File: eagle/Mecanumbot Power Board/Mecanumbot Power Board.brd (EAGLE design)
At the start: 100.1 x 74.1 mm, 103 parts, among them J1 AVR_SPI_PRG_6PTH, U1 FT232RL-BASICSSOP, U2 ATMEGA168, X1 USBSMD, Y1 RESONATORSMD

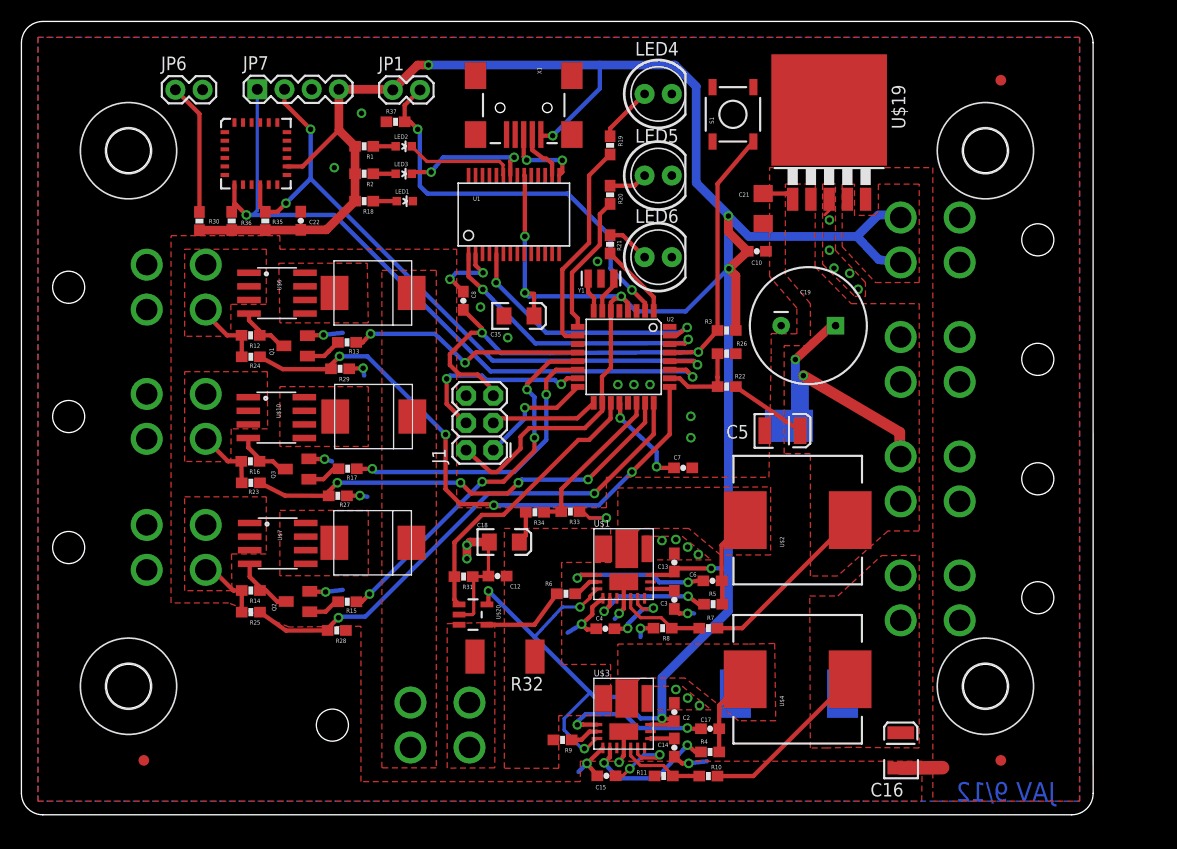
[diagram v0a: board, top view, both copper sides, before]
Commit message: pushing back v2.0 from svn
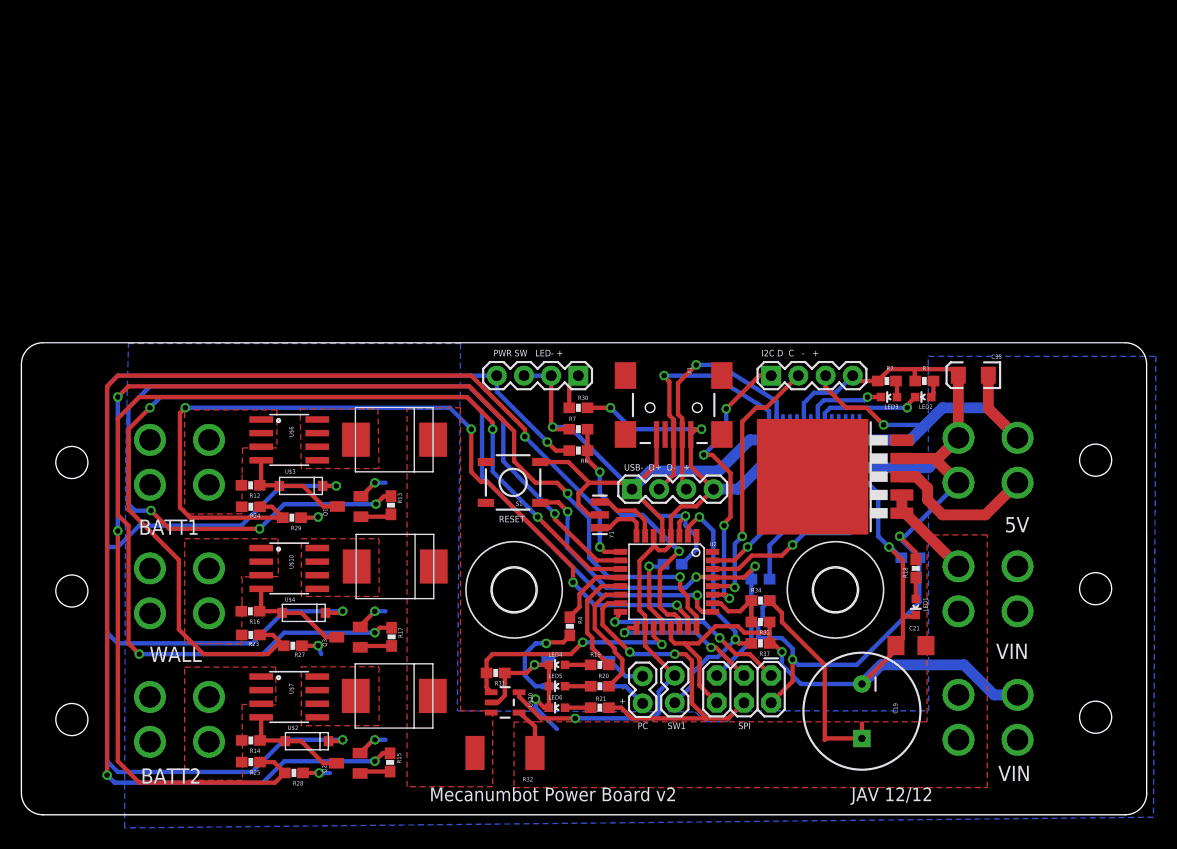
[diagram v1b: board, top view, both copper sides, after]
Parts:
- removed C12, C13, C14, C17, C2, C3, C6: 1uF, SparkFun:0603-CAP
- removed C15, C22, C4: 0.1uF, SparkFun:0603-CAP
- removed C16, C5: 330uF, SparkFun:EIA3528
- removed C18: 68uF, SparkFun:EIA3216
- removed JP4: FIDUCIAL1X2.5, SparkFun:FIDUCIAL-1X2.5
- removed JP6: PWR LED, SparkFun:1X02
- removed R10: 24K, SparkFun:0603-RES
- removed R11, R8: 1K, SparkFun:0603-RES
- removed R22: 10K, SparkFun:0603-RES
- removed R26: 3.3K, SparkFun:0603-RES
- removed R35, R36: 10k, SparkFun:0603-RES
- removed R5: 7.5K, SparkFun:0603-RES
- removed R9: 200K, SparkFun:0603-RES
- removed U$15, U$9: TERMINAL-4MINIFIT-JR, AT-Parts-RJ:MINIFITJR-RGT-4
- removed U$21: SUPERCAPS-LEAD, AT-Parts-RJ:AVX-SUPERCAP-S-LEAD
- removed U$22: HMC6352, SparkFun:LCC24
- removed U$23, U$25: (no value), holes:4,1
- added PC-CTRL: S2, SparkFun:1X02
- JP2: value FIDUCIAL1X2.5 -> USB; device SparkFun:FIDUCIAL-1X2.5 -> SparkFun:1X04
- JP3: value FIDUCIAL1X2.5 -> PWR-CTRL; device SparkFun:FIDUCIAL-1X2.5 -> SparkFun:1X04
- LED3: value Green -> Yellow
- LED4, LED5, LED6: value RED -> Blue; device SparkFun:LED5MM -> SparkFun:LED-0603
- R37: value 10k -> 10K
- R4: value 7.5K -> 330
- R6: value 200K -> 10K
- R7: value 24K -> 3.3K
- U$1: value IR3477 -> CLA230TR-NDSMD; device AT-Parts-RJ:IR3477 -> jav-parts:4-SOP
- U$2, U$4: value 1uH -> BZT52C33-FDICT-ND; device SparkFun:CDRH125 -> jav-parts:SOD-123
- U$3: value IR3477 -> BZT52C33-FDICT-ND; device AT-Parts-RJ:IR3477 -> jav-parts:SOD-123
- moved R18 61.9 mm to (83.5, 23.0), turned to 90 degrees
- moved LED1 60.9 mm to (83.5, 19.4), turned to 180 degrees
- moved JP1 60.7 mm to (61.0, 13.0), turned to 270 degrees
- moved R37 59.4 mm to (69.0, 16.0), turned to 180 degrees
- moved R1 56.7 mm to (84.3, 40.5)
- moved JP7 54.9 mm to (70.0, 41.0)
- moved U$26 54.6 mm to (46.0, 21.0)
- moved LED4 54.1 mm to (50.0, 14.0), turned to 90 degrees
- moved LED2 53.9 mm to (84.2, 39.0), turned to 90 degrees
- moved JP3 53.3 mm to (52.0, 41.0), turned to 180 degrees
- moved R2 52.5 mm to (80.8, 40.5)
- moved JP2 52.1 mm to (57.0, 30.4)
- moved U$2 50.3 mm to (26.6, 6.87), turned to 0 degrees
- moved LED3 49.9 mm to (81.0, 39.0), turned to 90 degrees
- moved LED5 48.6 mm to (50.0, 12.0), turned to 90 degrees
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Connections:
- removed net 12VA: C19.1, C21.1, C5.A, R22.2, R7.2, U$15.3, U$15.4, U$17.3, U$17.4, U$19.1, U$19.2, U$2.2, U$21.PLUS1
- removed net 12VB: C16.A, R10.2, U$16.3, U$16.4, U$4.2
- removed net N$17: R4.1, U$3.2
- removed net N$18: C3.2, U$1.8
- removed net N$19: R6.1, U$1.15
- removed net N$21: R10.1, R11.2, U$3.5
- removed net N$22: C14.2, U$3.8
- removed net N$23: R9.1, U$3.15
- removed net N$24: C15.2, U$3.6
- removed net N$25: C4.2, U$1.6
- removed net N$35: R19.2, U2.10
- removed net N$36: R20.2, U2.9
- removed net N$37: R21.2, U2.1
- removed net N$41: R22.1, R26.2, U2.26
- removed net N$45: JP6.1, R30.2
- removed net POST-DIODE: U$11.P$1, U$5.P$1, U$8.P$1, U$9.1, U$9.2
- new net N$14: R20.2, U2.14
- new net PCCTRL: R4.1, U2.12
- new net PWRSW: JP3.4, R6.2, U$2.CA, U$3.CA, U$4.CA
- net BATT1EN: now also U2.10; no longer U2.12
- net BATT2EN: now also U2.9; no longer U2.13
- net GND: now also JP2.1, JP3.2, JP3.3, LED4.C, LED5.C, LED6.C, R7.1, S1.3, U$1.2; no longer C12.2, C13.2, C14.1, C15.1, C16.C, C18.C, C2.2, C22.2, C3.1, C4.1, C5.C, JP6.2, LED4.K, LED5.K, LED6.K, R11.1, R26.1, R8.1, S1.1, U$1.1, U$1.11, U$1.17, U$1.4, U$15.1, U$15.2, U$21.MINUS1, U$21.MINUS2, U$22.5, U$3.1, U$3.11, U$3.17, U$3.4
- net MOSI: now also R21.2
- net N$12: now also R4.2, U$1.1; no longer R5.1, U$1.2
- net N$13: now also JP3.1, R30.2; no longer C17.1, U$3.14
- net N$15: now also R33.2, R34.1, U2.26; no longer C17.2, R4.2, U$3.12, U$4.1
- net N$16: now also R19.2, U2.13; no longer R7.1, R8.2, U$1.5
- net N$26: now also U$3.AN
- net N$29: now also U$2.AN
- net N$32: now also U$4.AN
- net N$42: now also U2.25; no longer U2.23
- net N$44: now also U2.23; no longer U2.25
- net N$46: now also R6.1, R7.2; no longer R33.2, R34.1
- net N$5: now also PC-CTRL.2, U$1.3; no longer C6.1, U$1.14
- net N$6: now also PC-CTRL.1, U$1.4; no longer C6.2, R5.2, U$1.12, U$2.1
- net N$7: now also JP2.3
- net N$8: now also JP2.2
- net PRE-VIN: now also U$11.P$1, U$5.P$1, U$8.P$1; no longer U$9.3, U$9.4
- net RESET: now also S1.1; no longer S1.3
- net SCL: no longer R35.1, U$22.10
- net SDA: no longer R36.1, U$22.7
- net VCC: now also JP2.4; no longer C13.1, C2.1, C22.1, R35.2, R36.2, U$1.10, U$1.16, U$22.14, U$3.10, U$3.16
- net VIN: now also C19.1, C21.1, U$16.3, U$16.4, U$17.3, U$17.4, U$19.1, U$19.2; no longer C12.1, C18.A, R6.2, R9.2, U$1.13, U$3.13
- net WALLPWREN: now also U2.11; no longer U2.14
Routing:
- net GND: track 61.0 -> 254.2 mm, vias 37 -> 13
- net PWRSW: track 0.00 -> 157.7 mm, vias 0 -> 4
- net VCC: track 290.9 -> 169.9 mm, vias 12 -> 5
- net BATT2EN: track 34.6 -> 121.7 mm
- net WALLPWREN: track 28.0 -> 104.5 mm, vias 2 -> 4
- net N$43: track 47.9 -> 123.2 mm, vias 2 -> 4
- net BATT1EN: track 22.5 -> 91.7 mm, vias 2 -> 4
- net N$42: track 42.0 -> 102.8 mm, vias 4 -> 2
- net 12VA: track 55.1 -> 0.00 mm, vias 2 -> 0
- net SCL: track 63.6 -> 24.9 mm, vias 3 -> 2
- net SDA: track 66.4 -> 27.9 mm, vias 2 -> 4
- net N$44: track 55.2 -> 81.3 mm
- net VIN: track 11.0 -> 33.6 mm
- net RESET: track 58.6 -> 37.9 mm, vias 2 -> 3
- net N$35: track 20.1 -> 0.00 mm
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- removed copper zone on layer 1, net 12VA
- removed copper zone on layer 1, net 12VB
- removed copper zone on layer 1, net GND
- removed copper zone on layer 1, net N$15
- removed copper zone on layer 1, net N$6
- removed copper zone on layer 1, net POST-DIODE
- removed copper zone on layer 1, net VCC
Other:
- board size 100.1 x 74.1 mm -> 105.1 x 44.1 mm
- board text added: "+ -"
- board text added: "BATT1"
- board text added: "BATT2"
- board text added: "I2C D C - +"
- board text added: "JAV 12/12"
- board text added: "Mecanumbot Power Board v2"
- board text added: "PWR SW LED- +"
- board text added: "RESET"
- board text added: "SPI"
- board text added: "SW1"
- board text added: "USB- D+ D- +"
- board text added: "VIN"
- board text removed: "+ - C D"
- board text removed: "- +"
- board text removed: "12V"
- board text removed: "B1"
- board text removed: "B2"
- board text removed: "I2C"
- board text removed: "JAV 9/12"
- board text removed: "LED"
- board text removed: "MTR"
- board text removed: "Mecanumbot Power Board v1"
- board text removed: "PWR"
- board text removed: "RST"
- board text removed: "SW2"
